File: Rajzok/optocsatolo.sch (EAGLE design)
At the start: 17 parts, among them Q1 TP0602N2, Q2 TP0602N2, Q3 SUP75N06-08, Q4 SUP75N06-08

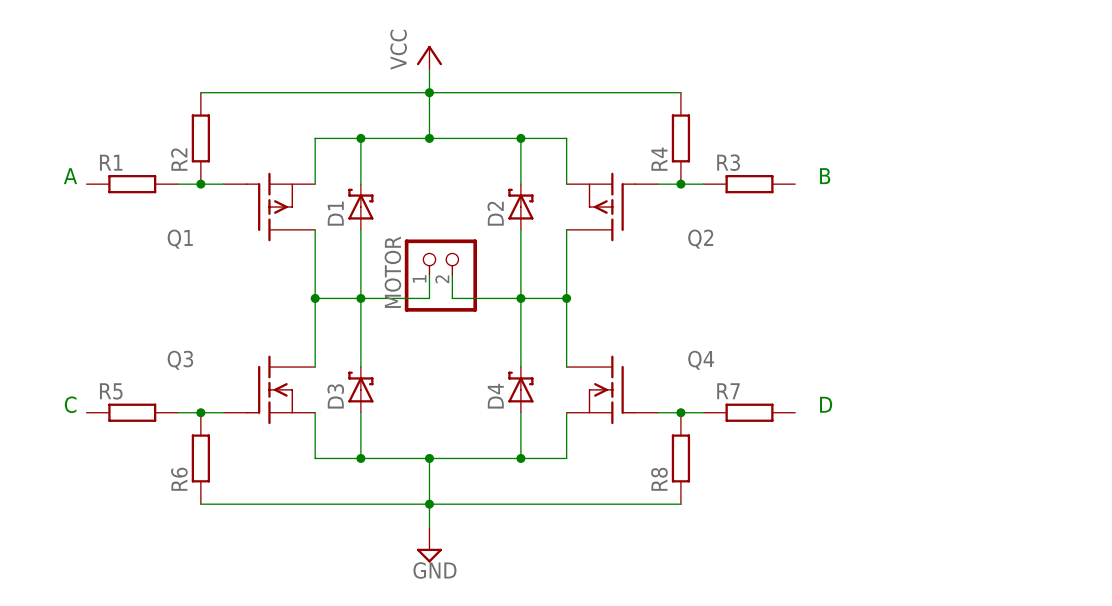
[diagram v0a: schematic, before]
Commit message: Rajzok 2017
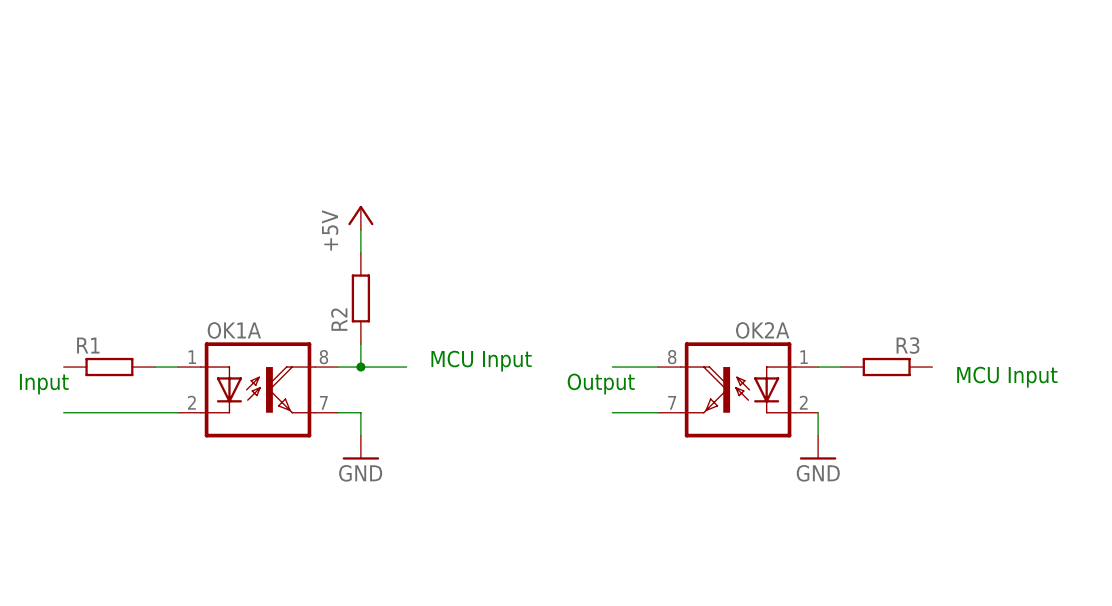
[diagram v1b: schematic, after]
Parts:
- removed D1, D2, D3, D4: 1N6267A, diode:1N6267A
- removed MOTOR: (no value), pinhead:PINHD-1X2
- removed Q1, Q2: TP0602N2, transistor-fet:TP0602N2
- removed Q3, Q4: SUP75N06-08, transistor-fet:SUP75N06-08
- removed R4, R5, R6, R7, R8: (no value), rcl:R-EU_0204/7
- added OK1, OK2: TIL198, optocoupler:TIL198
- R1, R2, R3: device rcl:R-EU_0204/7 -> resistor:R-EU_R1206W
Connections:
- removed net N$9: D1.A, D3.C, MOTOR.1, Q1.D, Q3.D
- removed net VCC: D1.C, D2.C, Q1.S, Q2.S, R2.2, R4.2
- new net +5V: R2.2
- new net N$6: OK2A.COL
- net GND: now also OK1A.EMI, OK2A.C; no longer D3.A, D4.A, Q3.S, Q4.S, R6.1, R8.1
- net N$1: now also OK1A.COL; no longer Q1.G, R1.2
- net N$2: now also OK2A.EMI; no longer D2.A, D4.C, MOTOR.2, Q2.D, Q4.D
- net N$3: now also OK1A.A, R1.2; no longer Q2.G, R3.1, R4.1
- net N$4: now also OK1A.C; no longer Q3.G, R5.2, R6.2
- net N$5: now also OK2A.A, R3.2; no longer Q4.G, R7.1, R8.2
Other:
- note added: "Input"
- note added: "MCU Input"
- note added: "Output"
- note removed: "A"
- note removed: "B"
- note removed: "C"
- note removed: "D"
- moved on the sheet: R1, R2, R3
